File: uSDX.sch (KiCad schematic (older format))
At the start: 27 parts, among them J1 Jack-DC, J2 GPS_CONN, J3 ICSP, J4 SMA, U1 L7805, U2 LD1117S33TR_SOT223, U3 ATmega328PB-AU, Y1 20MHz

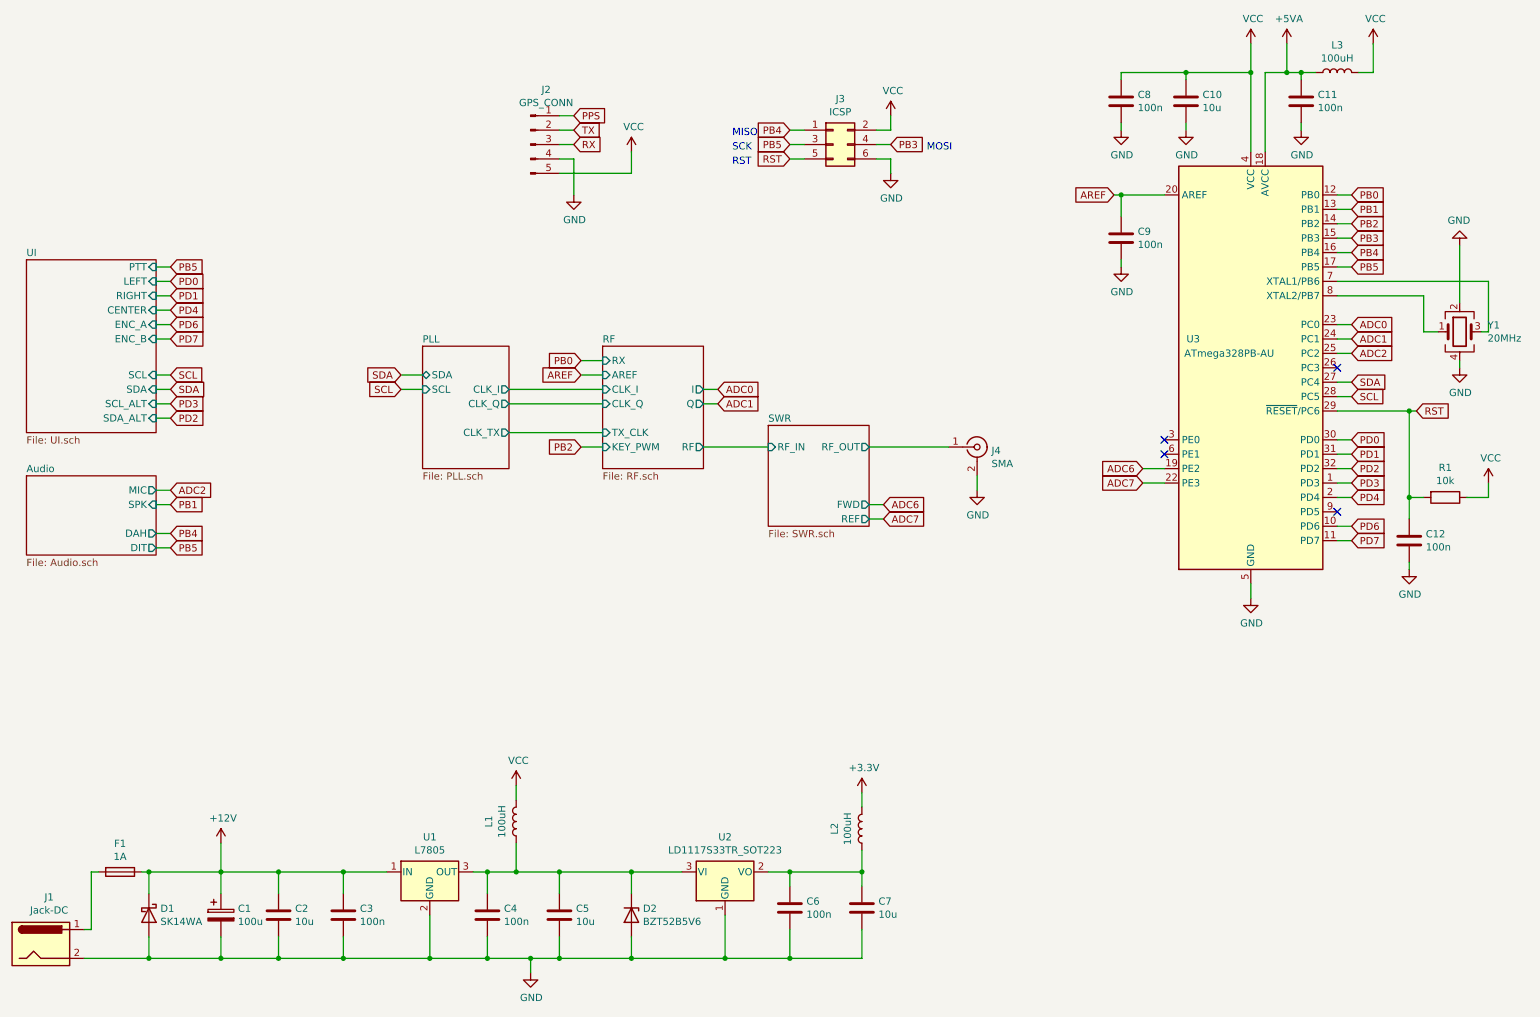
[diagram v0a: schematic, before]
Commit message: Almost final PCB
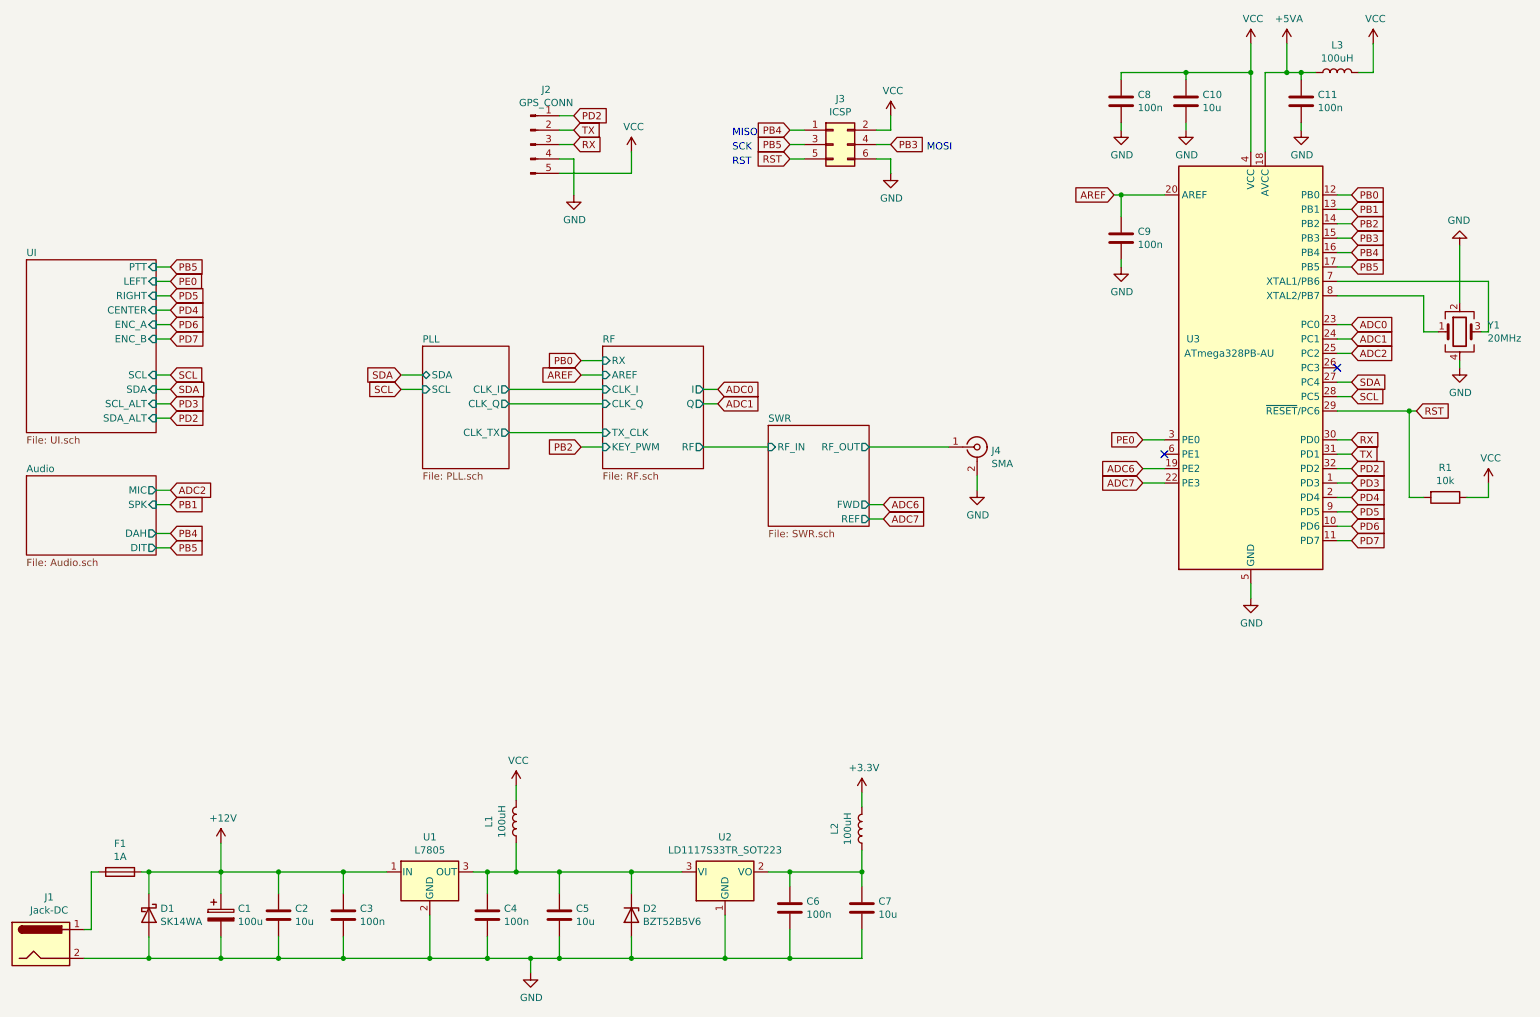
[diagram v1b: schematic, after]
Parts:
- removed C12: 100n, Capacitor_SMD:C_0805_2012Metric_Pad1.18x1.45mm_HandSolder, symbol Device:C
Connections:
- net PD0 is gone; now on net RX: U3.30 (PD0)
- net PD1 is gone; now on net TX: U3.31 (PD1)
- net PPS is gone; now on net PD2: J2.1 (Pin_1)
- net PE0: now reaches U3.3 (PE0)
- net PD5: now reaches U3.9 (PD5)
- no-connect marks 4 -> 2
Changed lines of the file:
@@
 	1    0    0    -1
 $EndComp
-Text GLabel 4500 1350 2    50   Input ~ 0
-PPS
 Text GLabel 4500 1550 2    50   Input ~ 0
 RX
@@
 Wire Wire Line
 	6650 4150 6550 4150
-Text GLabel 9900 3600 2    50   Input ~ 0
-PD0
-Text GLabel 9900 3700 2    50   Input ~ 0
-PD1
 Text GLabel 9900 4000 2    50   Input ~ 0
 PD4
-Text GLabel 1700 2500 2    50   Input ~ 0
-PD0
-Text GLabel 1700 2600 2    50   Input ~ 0
-PD1
 Text GLabel 1700 2700 2    50   Input ~ 0
 PD4
@@
 Wire Wire Line
 	9800 4000 9900 4000
-NoConn ~ 8600 3600
 NoConn ~ 8600 3700
 Text GLabel 9900 2200 2    50   Input ~ 0
@@
 Connection ~ 10300 3400
 $Comp
-L Device:C C12
-U 1 1 60E67CD4
-P 10300 4300
-F 0 "C12" H 10185 4254 50  0000 R CNN
-F 1 "100n" H 10185 4345 50  0000 R CNN
-F 2 "Capacitor_SMD:C_0805_2012Metric_Pad1.18x1.45mm_HandSolder" H 10338 4150 50  0001 C CNN
-F 3 "~" H 10300 4300 50  0001 C CNN
-	1    10300 4300
-	-1   0    0    1
-$EndComp
-Wire Wire Line
-	10300 4150 10300 4000
-Connection ~ 10300 4000
-$Comp
-L power:GND #PWR018
-U 1 1 60E704DF
-P 10300 4500
-F 0 "#PWR018" H 10300 4250 50  0001 C CNN
-F 1 "GND" H 10305 4327 50  0000 C CNN
-F 2 "" H 10300 4500 50  0001 C CNN
-F 3 "" H 10300 4500 50  0001 C CNN
-	1    10300 4500
-	1    0    0    -1
-$EndComp
-Wire Wire Line
-	10300 4500 10300 4450
-NoConn ~ 9800 4100
-$Comp
 L Device:Crystal_GND24 Y1
 U 1 1 610588A8
@@
 Wire Wire Line
 	10650 2250 10650 2650
+Text GLabel 9900 3600 2    50   Input ~ 0
+RX
+Text GLabel 9900 3700 2    50   Input ~ 0
+TX
+Text GLabel 4500 1350 2    50   Input ~ 0
+PD2
+Text GLabel 9900 4100 2    50   Input ~ 0
+PD5
+Wire Wire Line
+	9900 4100 9800 4100
+Text GLabel 1700 2600 2    50   Input ~ 0
+PD5
+Text GLabel 8450 3600 0    50   Input ~ 0
+PE0
+Wire Wire Line
+	8450 3600 8600 3600
+Text GLabel 1700 2500 2    50   Input ~ 0
+PE0
 $EndSCHEMATC
